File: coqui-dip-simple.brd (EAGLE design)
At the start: 48 x 13 mm, 29 parts, among them IC3 MCP73831, IC4 MCP1700-33, J1 AYZ0202, X1 USBSMD

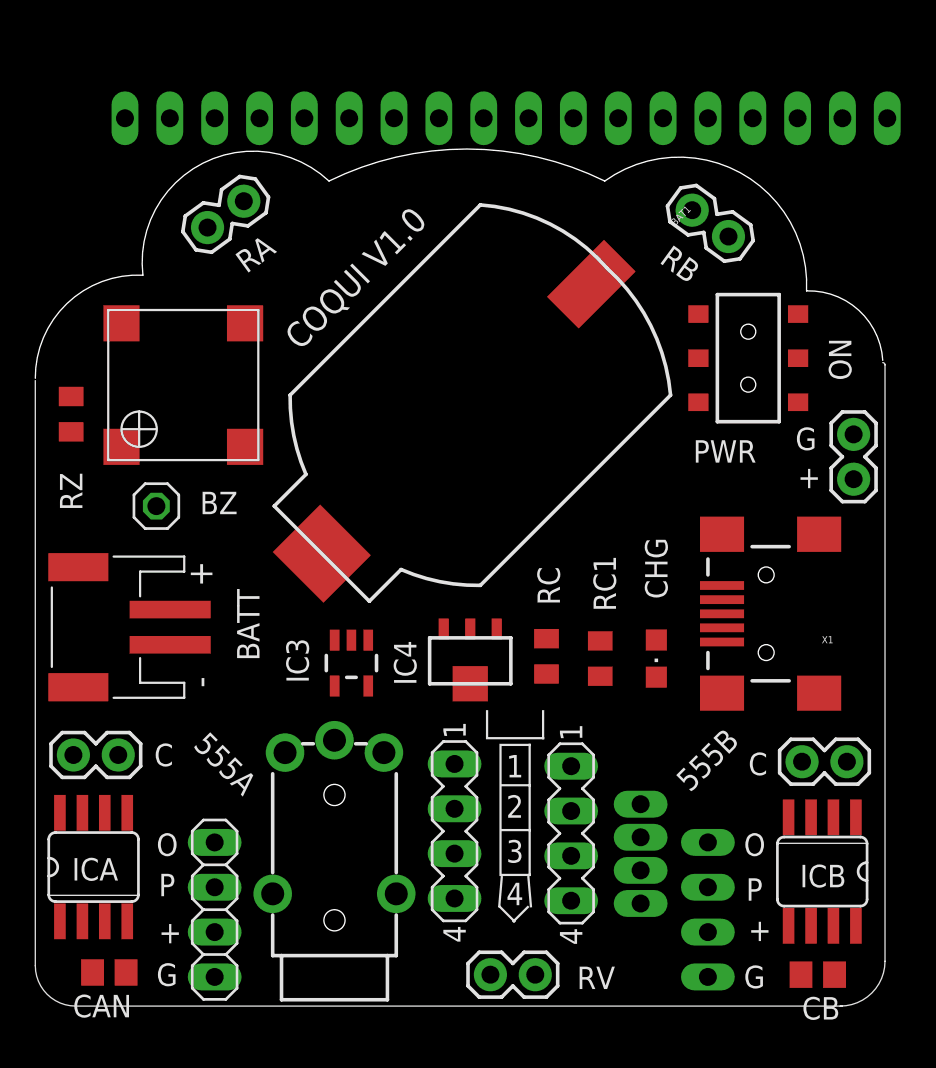
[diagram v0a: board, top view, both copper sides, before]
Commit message: update
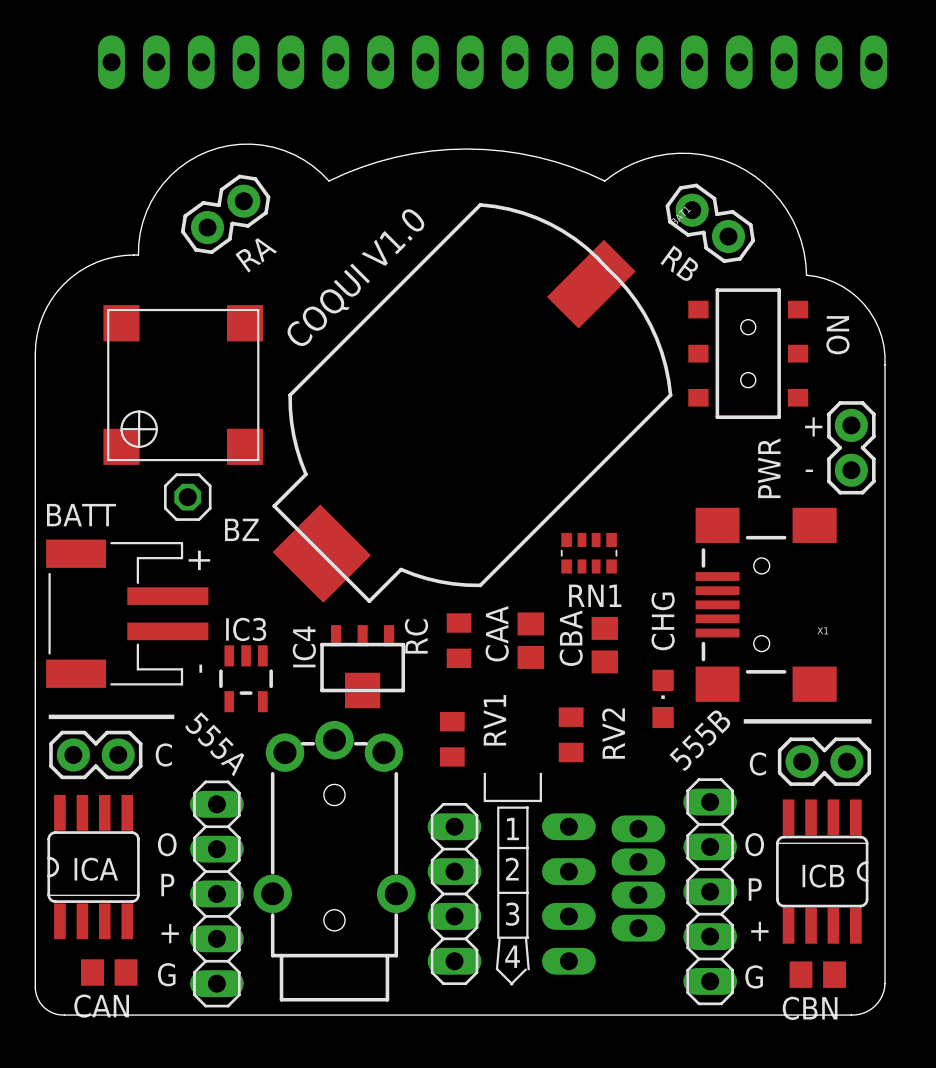
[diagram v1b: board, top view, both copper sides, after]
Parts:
- removed C2, RV: M02PTH, SparkFun-Connectors:1X02
- removed JACK, JACK1: (no value), con-lstb:MA04-1
- removed RC1: 4.7K, adafruit2013:R0805
- removed RZ: 1, adafruit2013:R0805
- added CAA, CBA, CBN: 0.01uF, rcl:C0805
- added JP5, JP6: (no value), pinhead:1X05
- added RN1: (no value), resistor-dil:EXB38V
- added RV1, RV2: 22K, adafruit2013:R0805
- CAN: device rcl:C0805@1 -> rcl:C0805
- CB: value 0.01uF -> M02PTH; device rcl:C0805@1 -> SparkFun-Connectors:1X02
- RC: value 4.7K -> 22K
- moved JP4 13.6 mm to (22.7, 6.22)
- moved CB 12.2 mm to (45.0, 13.7)
- moved JP3 7.92 mm to (29.2, 6.22)
- moved IC4 6.11 mm to (17.5, 19.1)
- moved IC3 6.03 mm to (10.9, 18.4)
- moved RC 5.03 mm to (23.0, 20.6), turned to 90 degrees
- moved JP2 3.27 mm to (24.9, 53.3)
- moved CHG 2.32 mm to (34.5, 17.3), turned to 0 degrees
- moved BZ 1.85 mm to (7.62, 28.7)
- moved JP1 1.40 mm to (30.9, 6.99)
- moved BATT 0.77 mm to (2.79, 22.1)
- moved X1 0.57 mm to (40.1, 22.6)
- moved PWR 0.52 mm to (45.2, 32.8)
- moved J1 0.25 mm to (39.4, 36.8)
- renumbered C1 to CA
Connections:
- removed net V+: ICA.8, ICB.8
- new net AOUT: ICB.3, JP5.5, RA.2, RN1.3, RV1.2
- new net BOUT: JP6.5, RB.2, RN1.4, RV2.2
- new net N$10: CAA.2, RV1.1
- new net N$11: CA.2, ICB.2, ICB.6, RA.1
- new net N$13: CBA.2, RV2.1
- new net N$14: CAN.2, ICB.5
- new net N$15: CBN.2, ICA.5
- new net N$16: CB.2, ICA.2, ICA.6, RB.1
- new net N$17: CBA.1, JP6.4
- new net N$18: JP1.1, JP3.1
- new net N$19: JP1.2, JP3.2
- new net N$20: JP1.3, JP3.3
- new net N$21: JP1.4, JP3.4
- new net N$9: CAA.1, JP5.4
- new net VAIN: ICB.4, ICB.8, JP5.3
- new net VBIN: ICA.4, ICA.8, JP6.3
- net GND: now also CA.1, CAN.1, CB.1, CBN.1, JP5.1, JP6.1, PWR.2, RN1.5, RN1.6, X1.GND; no longer J-FEMALE.3
- net N$1: now also J-FEMALE.1, JP4.1; no longer J-FEMALE.4
- net N$12: now also RN1.2; no longer RZ.1
- net N$2: now also JP4.2; no longer JP1.1
- net N$4: now also J-FEMALE.3, JP4.3; no longer X1.GND
- net N$6: now also J-FEMALE.4, JP4.4; no longer J-FEMALE.1
- net N$7: now also RN1.7; no longer RZ.2
- net N$8: now also RN1.1; no longer RC1.1
- net VBUS: now also RN1.8; no longer RC1.2
- net VCC: now also JP5.2, JP6.2
- net VDD: now also PWR.1
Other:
- board size 48 x 13 mm -> 48.1 x 49.3 mm
- board text added: "-"
